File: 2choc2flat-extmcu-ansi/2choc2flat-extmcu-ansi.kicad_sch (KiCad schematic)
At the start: 140 parts, among them J1 Conn_01x09_Male, J2 Conn_01x05_Male, J3 Conn_01x09_Male, K1 KEYSW, K10 KEYSW, K11 KEYSW, K12 KEYSW, K13 KEYSW, K14 KEYSW, K16 KEYSW, K17 KEYSW, K18 KEYSW, K19 KEYSW, K2 KEYSW, K20 KEYSW, K21 KEYSW, K22 KEYSW, K23 KEYSW, K24 KEYSW, K25 KEYSW, K26 KEYSW, K27 KEYSW, K28 KEYSW, K29 KEYSW, K3 KEYSW, K31 KEYSW, K31-1 KEYSW, K32 KEYSW, K33 KEYSW, K34 KEYSW, K35 KEYSW, K36 KEYSW, K37 KEYSW, K38 KEYSW, K39 KEYSW, K4 KEYSW, K40 KEYSW, K41 KEYSW, K42 KEYSW, K44 KEYSW, K46 KEYSW, K47 KEYSW, K48 KEYSW, K49 KEYSW, K5 KEYSW, K50 KEYSW, K51 KEYSW, K52 KEYSW, K53 KEYSW, K54 KEYSW, K55 KEYSW, K56 KEYSW, K57 KEYSW, K58 KEYSW, K59 KEYSW, K6 KEYSW, K61 KEYSW, K62 KEYSW, K63 KEYSW, K67 KEYSW, K7 KEYSW, K71 KEYSW, K72 KEYSW, K73 KEYSW, K74 KEYSW, K75 KEYSW, K8 KEYSW, K9 KEYSW

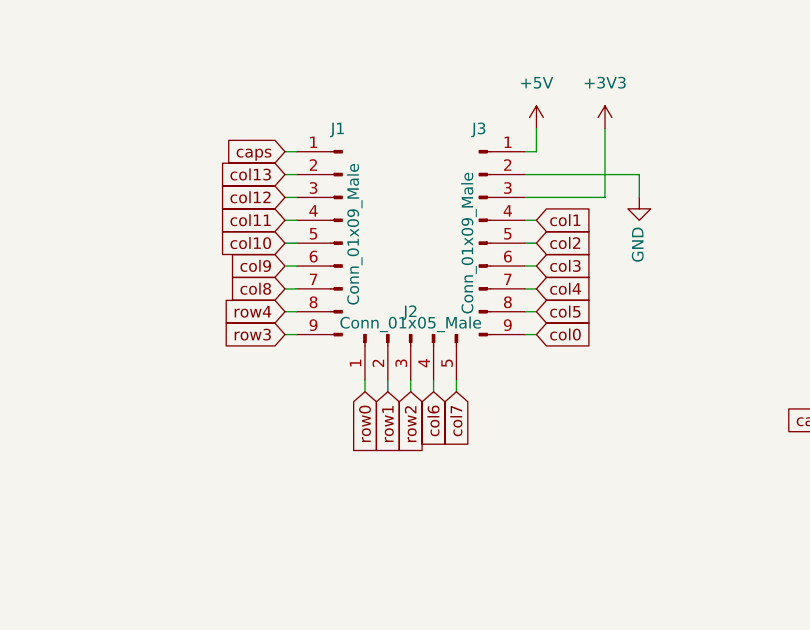
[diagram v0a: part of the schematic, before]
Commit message: routing complete
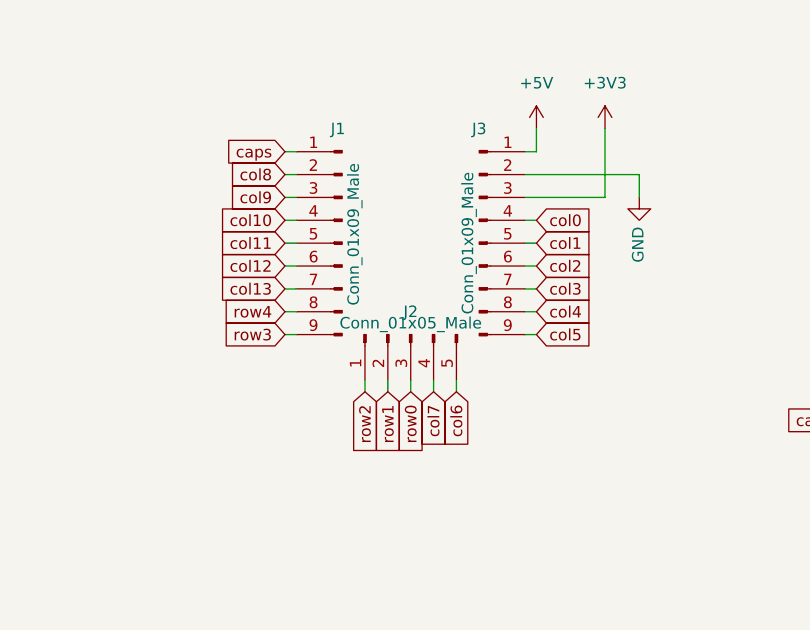
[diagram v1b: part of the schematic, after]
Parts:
- S3: footprint MountingHole:MountingHole_2.2mm_M2_Pad_Via -> MountingHole:MountingHole_2.2mm_M2_Pad_TopOnly
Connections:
- net col0: now also J3.4 (Pin_4); no longer J3.9 (Pin_9)
- net col1: now also J3.5 (Pin_5); no longer J3.4 (Pin_4)
- net col10: now also J1.4 (Pin_4); no longer J1.5 (Pin_5)
- net col11: now also J1.5 (Pin_5); no longer J1.4 (Pin_4)
- net col12: now also J1.6 (Pin_6); no longer J1.3 (Pin_3)
- net col13: now also J1.7 (Pin_7); no longer J1.2 (Pin_2)
- net col2: now also J3.6 (Pin_6); no longer J3.5 (Pin_5)
- net col3: now also J3.7 (Pin_7); no longer J3.6 (Pin_6)
- net col4: now also J3.8 (Pin_8); no longer J3.7 (Pin_7)
- net col5: now also J3.9 (Pin_9); no longer J3.8 (Pin_8)
- net col6: now also J2.5 (Pin_5); no longer J2.4 (Pin_4)
- net col7: now also J2.4 (Pin_4); no longer J2.5 (Pin_5)
- net col8: now also J1.2 (Pin_2); no longer J1.7 (Pin_7)
- net col9: now also J1.3 (Pin_3); no longer J1.6 (Pin_6)
- net row0: now also J2.3 (Pin_3); no longer J2.1 (Pin_1)
- net row2: now also J2.1 (Pin_1); no longer J2.3 (Pin_3)

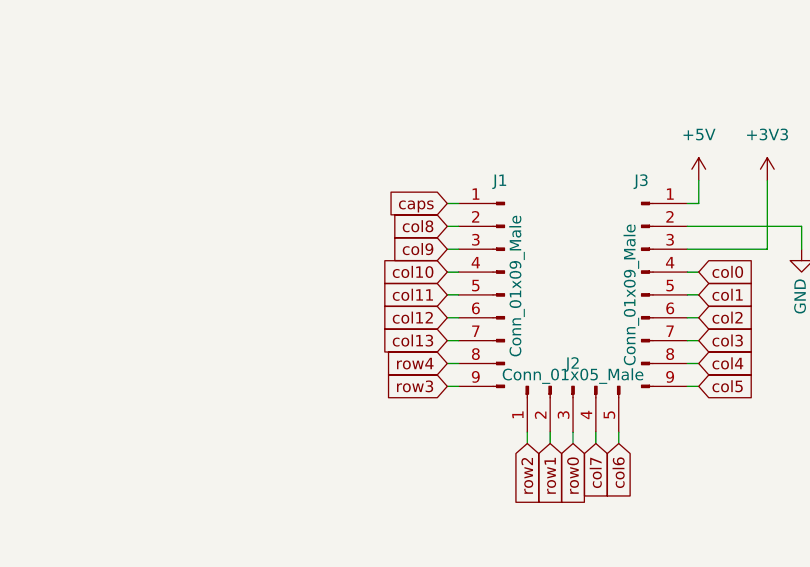
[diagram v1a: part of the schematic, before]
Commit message: rev 1.3 layouts
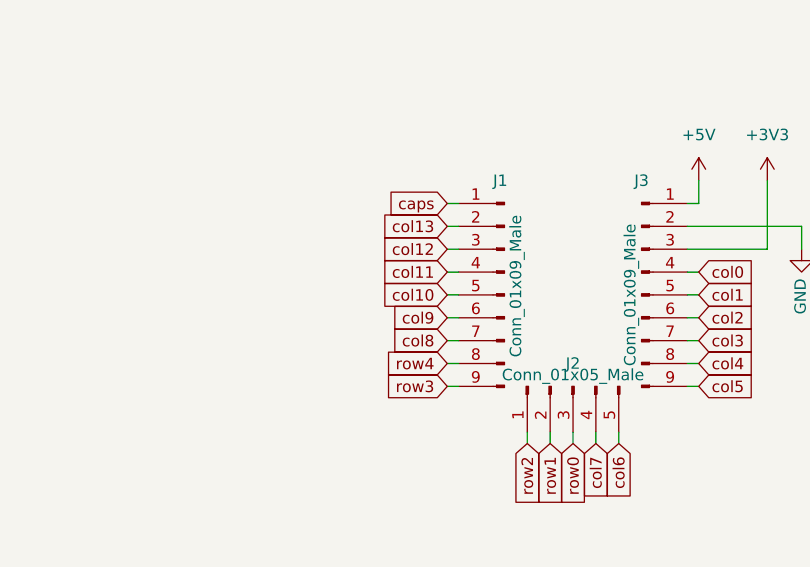
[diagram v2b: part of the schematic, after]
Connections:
- net col10: now also J1.5 (Pin_5); no longer J1.4 (Pin_4)
- net col11: now also J1.4 (Pin_4); no longer J1.5 (Pin_5)
- net col12: now also J1.3 (Pin_3); no longer J1.6 (Pin_6)
- net col13: now also J1.2 (Pin_2); no longer J1.7 (Pin_7)
- net col8: now also J1.7 (Pin_7); no longer J1.2 (Pin_2)
- net col9: now also J1.6 (Pin_6); no longer J1.3 (Pin_3)
